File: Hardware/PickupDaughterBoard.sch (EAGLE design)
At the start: 5 parts

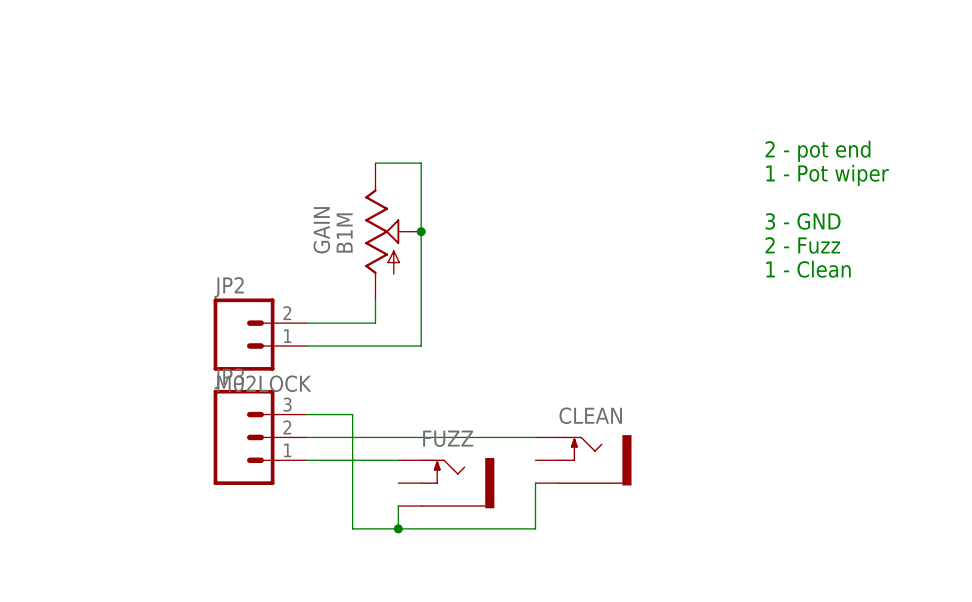
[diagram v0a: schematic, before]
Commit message: Designed and routed
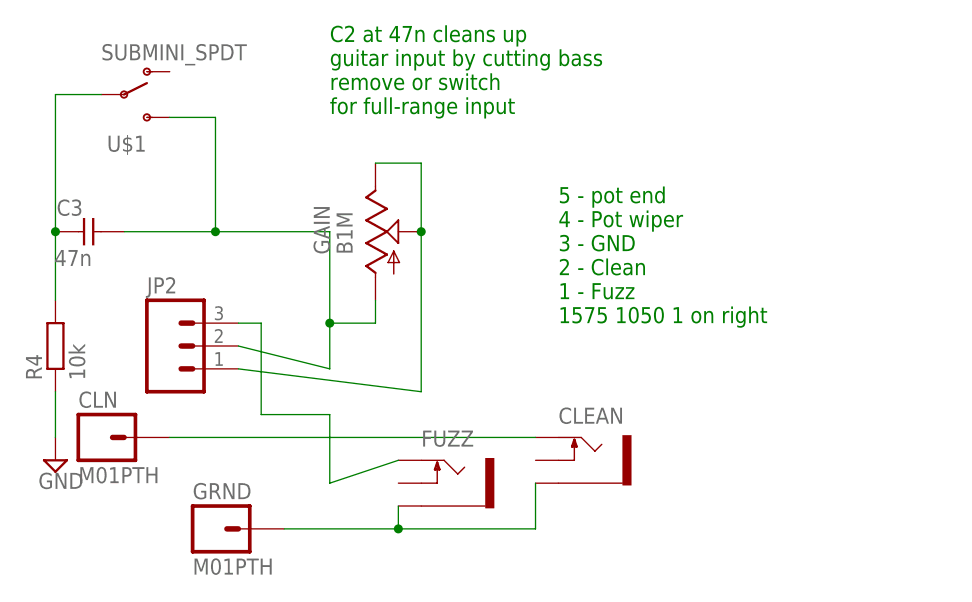
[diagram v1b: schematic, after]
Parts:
- removed JP3: (no value), SparkFun-Connectors:M03LOCK
- added C3: 47n, TomW:C-EU050-024X044
- added CLN, GRND: M01PTH, SparkFun-Connectors:M01PTH
- added R4: 10k, MusicThingModular:RESISTORVERTICAL
- added U$1: SUBMINI_SPDT, MusicThingModular:SUBMINI_SPDT
- JP2: value M02LOCK -> (none); device SparkFun-Connectors:M02LOCK -> SparkFun-Connectors:M03PTH
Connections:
- net N$8 renamed WIPER
- removed net N$1: FUZZ.TIP, JP3.1
- removed net N$2: CLEAN.TIP, JP3.2
- removed net N$4: GAIN.A, JP2.2
- new net CLEAN: CLEAN.TIP, CLN.1
- new net END: C3.1, GAIN.A, JP2.2, U$1.S
- new net FUZZ: FUZZ.TIP, JP2.3
- new net N$7: C3.2, R4.2, U$1.COMMON
- net GND: now also GRND.1, R4.1; no longer JP3.3
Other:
- note added: "5 - pot end 4 - Pot wiper 3 - GND 2 - Clean 1 - Fuzz 1575 1050 1 on right"
- note added: "C2 at 47n cleans up guitar input by cutting bass remove or switch for full-range input"
- note removed: "2 - pot end 1 - Pot wiper 3 - GND 2 - Fuzz 1 - Clean"
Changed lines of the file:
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@@
 <?xml version="1.0" encoding="utf-8"?>
 <!DOCTYPE eagle SYSTEM "eagle.dtd">
-<eagle version="7.4.0">
+<eagle version="7.7.0">
 <drawing>
 <settings>
@@
 <layer number="56" name="wert" color="7" fill="1" visible="no" active="no"/>
 <layer number="57" name="tCAD" color="7" fill="1" visible="no" active="no"/>
+<layer number="90" name="Modules" color="5" fill="1" visible="no" active="no"/>
 <layer number="91" name="Nets" color="2" fill="1" visible="yes" active="yes"/>
 <layer number="92" name="Busses" color="1" fill="1" visible="yes" active="yes"/>
@@
 <layer number="97" name="Info" color="7" fill="1" visible="yes" active="yes"/>
 <layer number="98" name="Guide" color="6" fill="1" visible="yes" active="yes"/>
+<layer number="99" name="SpiceOrder" color="5" fill="1" visible="no" active="no"/>
 <layer number="100" name="Muster" color="7" fill="1" visible="no" active="no"/>
 <layer number="101" name="Patch_Top" color="12" fill="4" visible="yes" active="yes"/>
@@
 </variantdefs>
 <classes>
-<class number="0" name="default" width="0.254" drill="0">
+<class number="0" name="default" width="0" drill="0">
 </class>
 <class number="1" name="power" width="0.4064" drill="0">
 </class>
-<class number="2" name="ground" width="0.4064" drill="0">
+<class number="2" name="ground" width="0.2032" drill="0">
 </class>
 </classes>
@@
 <part name="FRAME1" library="frames" deviceset="A4L-LOC" device=""/>
 <part name="FUZZ" library="MusicThingModular" deviceset="THONKICONN" device="NEW"/>
-<part name="JP2" library="SparkFun-Connectors" deviceset="M02" device="LOCK"/>
-<part name="JP3" library="SparkFun-Connectors" deviceset="M03" device="LOCK"/>
+<part name="U$1" library="MusicThingModular" deviceset="SUBMINI_SPDT" device=""/>
+<part name="R4" library="MusicThingModular" deviceset="RESISTOR" device="VERTICAL" value="10k"/>
+<part name="C3" library="TomW" deviceset="C-EU" device="050-024X044" value="47n"/>
+<part name="SUPPLY4" library="supply2" deviceset="GND" device=""/>
+<part name="JP2" library="SparkFun-Connectors" deviceset="M03" device="PTH"/>
+<part name="CLN" library="SparkFun-Connectors" deviceset="M01" device="PTH"/>
+<part name="GRND" library="SparkFun-Connectors" deviceset="M01" device="PTH"/>
 </parts>
 <sheets>
 <sheet>
 <plain>
-<text x="109.22" y="134.62" size="1.778" layer="91">2 - pot end
-1 - Pot wiper
+<text x="86.36" y="129.54" size="1.778" layer="91">5 - pot end
+4 - Pot wiper
 3 - GND
-2 - Fuzz
-1 - Clean</text>
+2 - Clean
+1 - Fuzz
+1575 1050 1 on right</text>
+<text x="60.96" y="162.56" size="1.778" layer="91" align="top-left">C2 at 47n cleans up
+guitar input by cutting bass
+remove or switch
+for full-range input </text>
 </plain>
 <instances>
@@
 <instance part="FRAME1" gate="G$1" x="0" y="0"/>
 <instance part="FUZZ" gate="G$1" x="73.66" y="111.76"/>
-<instance part="JP2" gate="G$1" x="50.8" y="127"/>
-<instance part="JP3" gate="G$1" x="50.8" y="116.84"/>
+<instance part="U$1" gate="G$1" x="40.64" y="154.94"/>
+<instance part="R4" gate="G$1" x="30.48" y="127" rot="R90"/>
+<instance part="C3" gate="G$1" x="35.56" y="139.7" rot="R270"/>
+<instance part="SUPPLY4" gate="GND" x="30.48" y="114.3"/>
+<instance part="JP2" gate="G$1" x="43.18" y="127"/>
+<instance part="CLN" gate="G$1" x="35.56" y="116.84"/>
+<instance part="GRND" gate="G$1" x="48.26" y="106.68"/>
 </instances>
 <busses>
 </busses>
 <nets>
-<net name="N$8" class="0">
+<net name="WIPER" class="0">
 <segment>
 <pinref part="GAIN" gate="G$1" pin="S"/>
@@
 <wire x1="71.12" y1="147.32" x2="71.12" y2="139.7" width="0.1524" layer="91"/>
 <wire x1="66.04" y1="147.32" x2="71.12" y2="147.32" width="0.1524" layer="91"/>
-<wire x1="71.12" y1="139.7" x2="71.12" y2="127" width="0.1524" layer="91"/>
+<wire x1="71.12" y1="139.7" x2="71.12" y2="121.92" width="0.1524" layer="91"/>
 <junction x="71.12" y="139.7"/>
-<wire x1="71.12" y1="127" x2="58.42" y2="127" width="0.1524" layer="91"/>
+<wire x1="71.12" y1="121.92" x2="50.8" y2="124.46" width="0.1524" layer="91"/>
 <pinref part="JP2" gate="G$1" pin="1"/>
 </segment>
 </net>
-<net name="N$1" class="0">
+<net name="FUZZ" class="0">
 <segment>
 <pinref part="FUZZ" gate="G$1" pin="TIP"/>
-<wire x1="68.58" y1="114.3" x2="58.42" y2="114.3" width="0.1524" layer="91"/>
-<pinref part="JP3" gate="G$1" pin="1"/>
-</segment>
-</net>
-<net name="N$2" class="0">
+<wire x1="68.58" y1="114.3" x2="60.96" y2="111.76" width="0.1524" layer="91"/>
+<wire x1="60.96" y1="111.76" x2="60.96" y2="119.38" width="0.1524" layer="91"/>
+<wire x1="60.96" y1="119.38" x2="53.34" y2="119.38" width="0.1524" layer="91"/>
+<wire x1="53.34" y1="119.38" x2="53.34" y2="129.54" width="0.1524" layer="91"/>
+<pinref part="JP2" gate="G$1" pin="3"/>
+<wire x1="53.34" y1="129.54" x2="50.8" y2="129.54" width="0.1524" layer="91"/>
+</segment>
+</net>
+<net name="CLEAN" class="0">
 <segment>
 <pinref part="CLEAN" gate="G$1" pin="TIP"/>
-<wire x1="58.42" y1="116.84" x2="83.82" y2="116.84" width="0.1524" layer="91"/>
-<pinref part="JP3" gate="G$1" pin="2"/>
+<wire x1="43.18" y1="116.84" x2="83.82" y2="116.84" width="0.1524" layer="91"/>
+<pinref part="CLN" gate="G$1" pin="1"/>
 </segment>
 </net>
 <net name="GND" class="0">
 <segment>
-<wire x1="58.42" y1="119.38" x2="63.5" y2="119.38" width="0.1524" layer="91"/>
-<wire x1="63.5" y1="119.38" x2="63.5" y2="106.68" width="0.1524" layer="91"/>
 <pinref part="CLEAN" gate="G$1" pin="SLEEVE"/>
-<wire x1="63.5" y1="106.68" x2="68.58" y2="106.68" width="0.1524" layer="91"/>
 <wire x1="68.58" y1="106.68" x2="83.82" y2="106.68" width="0.1524" layer="91"/>
 <wire x1="83.82" y1="106.68" x2="83.82" y2="111.76" width="0.1524" layer="91"/>
@@
 <wire x1="68.58" y1="109.22" x2="68.58" y2="106.68" width="0.1524" layer="91"/>
 <junction x="68.58" y="106.68"/>
-<pinref part="JP3" gate="G$1" pin="3"/>
-</segment>
-</net>
-<net name="N$4" class="0">
+<wire x1="68.58" y1="106.68" x2="55.88" y2="106.68" width="0.1524" layer="91"/>
+<pinref part="GRND" gate="G$1" pin="1"/>
+</segment>
+<segment>
+<pinref part="R4" gate="G$1" pin="1"/>
+<wire x1="30.48" y1="121.92" x2="30.48" y2="116.84" width="0.1524" layer="91"/>
+<pinref part="SUPPLY4" gate="GND" pin="GND"/>
+</segment>
+</net>
+<net name="END" class="0">
 <segment>
 <pinref part="GAIN" gate="G$1" pin="A"/>
 <wire x1="66.04" y1="132.08" x2="66.04" y2="129.54" width="0.1524" layer="91"/>
-<wire x1="66.04" y1="129.54" x2="58.42" y2="129.54" width="0.1524" layer="91"/>
+<wire x1="66.04" y1="129.54" x2="60.96" y2="129.54" width="0.1524" layer="91"/>
+<pinref part="C3" gate="G$1" pin="1"/>
+<wire x1="60.96" y1="129.54" x2="60.96" y2="124.46" width="0.1524" layer="91"/>
+<wire x1="60.96" y1="124.46" x2="50.8" y2="127" width="0.1524" layer="91"/>
+<wire x1="38.1" y1="139.7" x2="48.26" y2="139.7" width="0.1524" layer="91"/>
+<wire x1="48.26" y1="139.7" x2="60.96" y2="139.7" width="0.1524" layer="91"/>
+<wire x1="60.96" y1="139.7" x2="60.96" y2="129.54" width="0.1524" layer="91"/>
+<junction x="60.96" y="129.54"/>
+<pinref part="U$1" gate="G$1" pin="S"/>
+<wire x1="43.18" y1="152.4" x2="48.26" y2="152.4" width="0.1524" layer="91"/>
+<wire x1="48.26" y1="152.4" x2="48.26" y2="139.7" width="0.1524" layer="91"/>
+<junction x="48.26" y="139.7"/>
 <pinref part="JP2" gate="G$1" pin="2"/>
 </segment>
 </net>
+<net name="N$7" class="0">
+<segment>
+<pinref part="C3" gate="G$1" pin="2"/>
+<pinref part="R4" gate="G$1" pin="2"/>
+<wire x1="30.48" y1="139.7" x2="30.48" y2="132.08" width="0.1524" layer="91"/>
+<pinref part="U$1" gate="G$1" pin="COMMON"/>
+<wire x1="35.56" y1="154.94" x2="30.48" y2="154.94" width="0.1524" layer="91"/>
+<wire x1="30.48" y1="154.94" x2="30.48" y2="139.7" width="0.1524" layer="91"/>
+<junction x="30.48" y="139.7"/>
+</segment>
+</net>
